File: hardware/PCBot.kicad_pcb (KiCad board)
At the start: 4 copper layers, 68 x 37 mm, 101 parts, among them J101 Conn_ST_STDC14, M101 Motor_DC_ALT, M102 Motor_DC_ALT, U101 STM32G431CBUx, U102 AMS1117-3.3, U103 LSM6DS3, U104 STSPIN250, U105 STSPIN250, U201 A7105, Y101 Crystal_GND24_DNP, Y201 Crystal_GND24_DNP

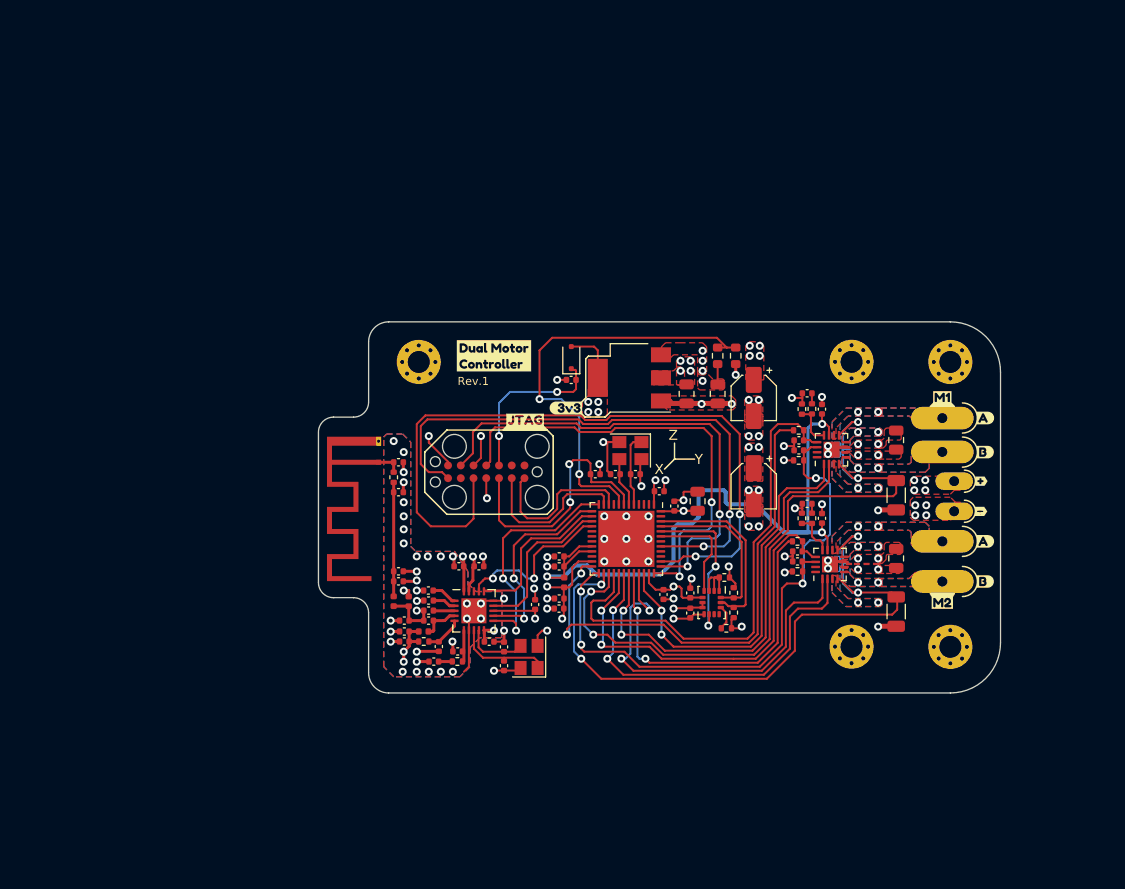
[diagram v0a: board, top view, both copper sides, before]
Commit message: initial commit 3
Signed-off-by: Connor Rigby <connorr@hey.com>
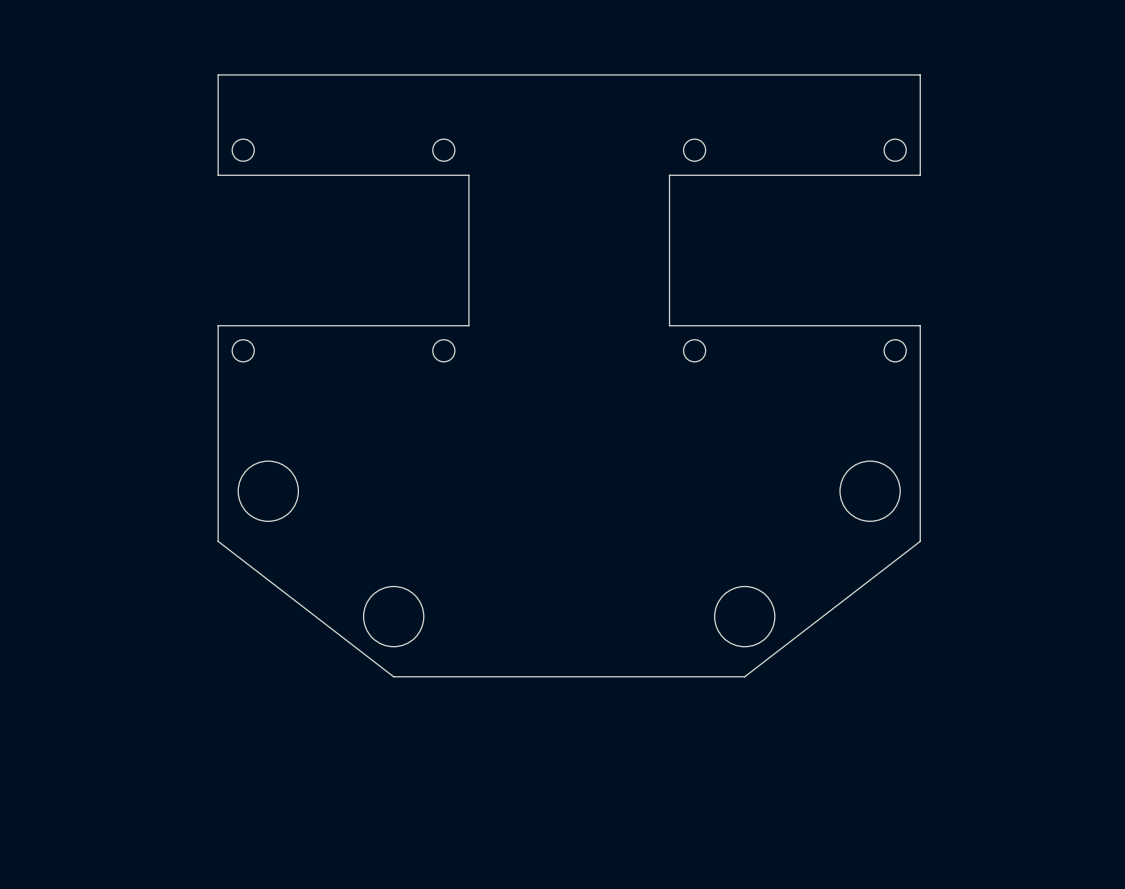
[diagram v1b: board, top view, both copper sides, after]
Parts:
- removed AE201: Antenna_Chip, RF_Antenna:Texas_SWRA117D_2.4GHz_Left
- removed BT101: Battery, LCSC_Connector:PAD_01x02
- removed C101, C102, C103, C109, C110, C114, C127, C128, C203, C206, C207, C208, C209, C211, C214, C215, C216, C217, C218, C219, C220: C_0402_DNP, Capacitor_SMD:C_0402_1005Metric
- removed C104, C111: C_0402_1nf_X7R, Capacitor_SMD:C_0402_1005Metric
- removed C105, C112: C_805_DNP, Capacitor_SMD:C_0805_2012Metric
- removed C106, C113: 22uf, Capacitor_SMD:CP_Elec_4x5.4
- removed C107: C_0805_1u_X7R, Capacitor_SMD:C_0805_2012Metric
- removed C108: C_0805_10u_X5R, Capacitor_SMD:C_0805_2012Metric
- removed C115, C116, C117, C118, C119, C122, C123, C124, C125, C126, C205: C_0402_100nf_X7R, Capacitor_SMD:C_0402_1005Metric
- removed C120: C_0805_4u7_X5R, Capacitor_SMD:C_0805_2012Metric
- removed C121: C_0402_1u_X5R, Capacitor_SMD:C_0402_1005Metric
- removed C201, C202, C204: C_0402_2u2_X5R, Capacitor_SMD:C_0402_1005Metric
- removed C210: C_0402_22p_C0G, Capacitor_SMD:C_0402_1005Metric
- removed C212: C_0402_100p_C0G, Capacitor_SMD:C_0402_1005Metric
- removed C213: C_0402_10n_C0G, Capacitor_SMD:C_0402_1005Metric
- removed D101: 30v 230mv@100ma 1A, Diode_SMD:D_SOD-323F
- removed FB101: FerriteBead_Small, Inductor_SMD:L_0402_1005Metric
- removed J101: Conn_ST_STDC14, LCSC_Connector:TC2070-IDC-FP
- removed L202, L203, L204: L_0402_DNP, Inductor_SMD:L_0402_1005Metric
- removed M101, M102: Motor_DC_ALT, LCSC_Connector:PAD_01x02
- removed R101, R102, R103, R106, R107, R110: 18k, Resistor_SMD:R_0402_1005Metric
- removed R104, R109, R113, R116: R_0402_1k, Resistor_SMD:R_0402_1005Metric
- removed R105, R108: R_1206_DNP, Resistor_SMD:R_1206_3216Metric
- removed R111, R112: R_0603_DNP, Resistor_SMD:R_0603_1608Metric
- removed R114, R115: R_0402_4k7, Resistor_SMD:R_0402_1005Metric
- removed R201, R203: DNP, Resistor_SMD:R_0402_1005Metric
- removed R202: 200, Resistor_SMD:R_0402_1005Metric
- removed REF** (x5): MountingHole_2.2mm_M2_Pad_Via, MountingHole:MountingHole_2.2mm_M2_Pad_Via
- removed U101: STM32G431CBUx, Package_DFN_QFN:QFN-48-1EP_7x7mm_P0.5mm_EP5.6x5.6mm
- removed U102: AMS1117-3.3, Package_TO_SOT_SMD:SOT-223-3_TabPin2
- removed U103: LSM6DS3, Package_LGA:LGA-14_3x2.5mm_P0.5mm_LayoutBorder3x4y
- removed U104, U105: STSPIN250, Package_DFN_QFN:TQFN-16-1EP_3x3mm_P0.5mm_EP1.6x1.6mm
- removed U201: A7105, Package_DFN_QFN:QFN-20-1EP_4x4mm_P0.5mm_EP2.5x2.5mm
- removed Y101, Y201: Crystal_GND24_DNP, Crystal:Crystal_SMD_3225-4Pin_3.2x2.5mm
- removed kibuzzard-646A62D2: G***, kibuzzard-646A62D2
- removed kibuzzard-646A6321: G***, kibuzzard-646A6321
- removed kibuzzard-646A63AE (x2): G***, kibuzzard-646A63AE
- removed kibuzzard-646A6533 (x2): G***, kibuzzard-646A6533
- removed kibuzzard-646A657B (x2): G***, kibuzzard-646A657B
- removed kibuzzard-646A6855: G***, kibuzzard-646A6855
- removed kibuzzard-646A6AA4: G***, kibuzzard-646A6AA4
- removed kibuzzard-646A6DD1: G***, kibuzzard-646A6DD1
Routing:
- net GND: track 90.8 -> 0.00 mm, vias 95 -> 0
- net /SYS_JTDI: track 72.9 -> 0.00 mm, vias 2 -> 0
- net /M2_SENSE: track 70.6 -> 0.00 mm, vias 4 -> 0
- net VDDA: track 67.8 -> 0.00 mm, vias 3 -> 0
- net /M1_SENSE: track 66.1 -> 0.00 mm, vias 4 -> 0
- net /MC_STBY_RESET: track 60.4 -> 0.00 mm, vias 4 -> 0
- net /SYS_JTDO: track 56.8 -> 0.00 mm, vias 2 -> 0
- net /M2_EN: track 51.9 -> 0.00 mm, vias 2 -> 0
- net /M2_EN_FAULT: track 50.7 -> 0.00 mm
- net VDD: track 48.6 -> 0.00 mm, vias 20 -> 0
- net /SYS_JTCK: track 48.2 -> 0.00 mm, vias 2 -> 0
- net /SYS_JTMS: track 45.8 -> 0.00 mm, vias 2 -> 0
- net /M2_PWM: track 43.6 -> 0.00 mm, vias 2 -> 0
- net /VBATT_SENSE: track 42.9 -> 0.00 mm, vias 2 -> 0
- net /M1_EN_FAULT: track 41.8 -> 0.00 mm, vias 2 -> 0
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- removed copper zone on F.Cu, net +BATT
- removed copper zone on B.Cu, net /M1_OUTA1
- removed copper zone on F.Cu, net /M1_OUTA1
- removed copper zone on B.Cu, net /M1_OUTA2
- removed copper zone on F.Cu, net /M1_OUTA2
- removed copper zone on B.Cu, net /M2_OUTA1
- removed copper zone on F.Cu, net /M2_OUTA1
- removed copper zone on B.Cu, net /M2_OUTA2
- removed copper zone on F.Cu, net /M2_OUTA2
- removed copper zone on B.Cu, net GND
- removed copper zone on F.Cu, net GND
- removed copper zone on F.Cu, net VDD
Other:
- board size 68 x 37 mm -> 70 x 60 mm
- board text removed: "Rev.1"
- board text removed: "X"
- board text removed: "Y"
- board text removed: "Z"

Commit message: uhhhhhhhhhhhhhhhhhhhhhhhh
Signed-off-by: Connor Rigby <connorr@hey.com>
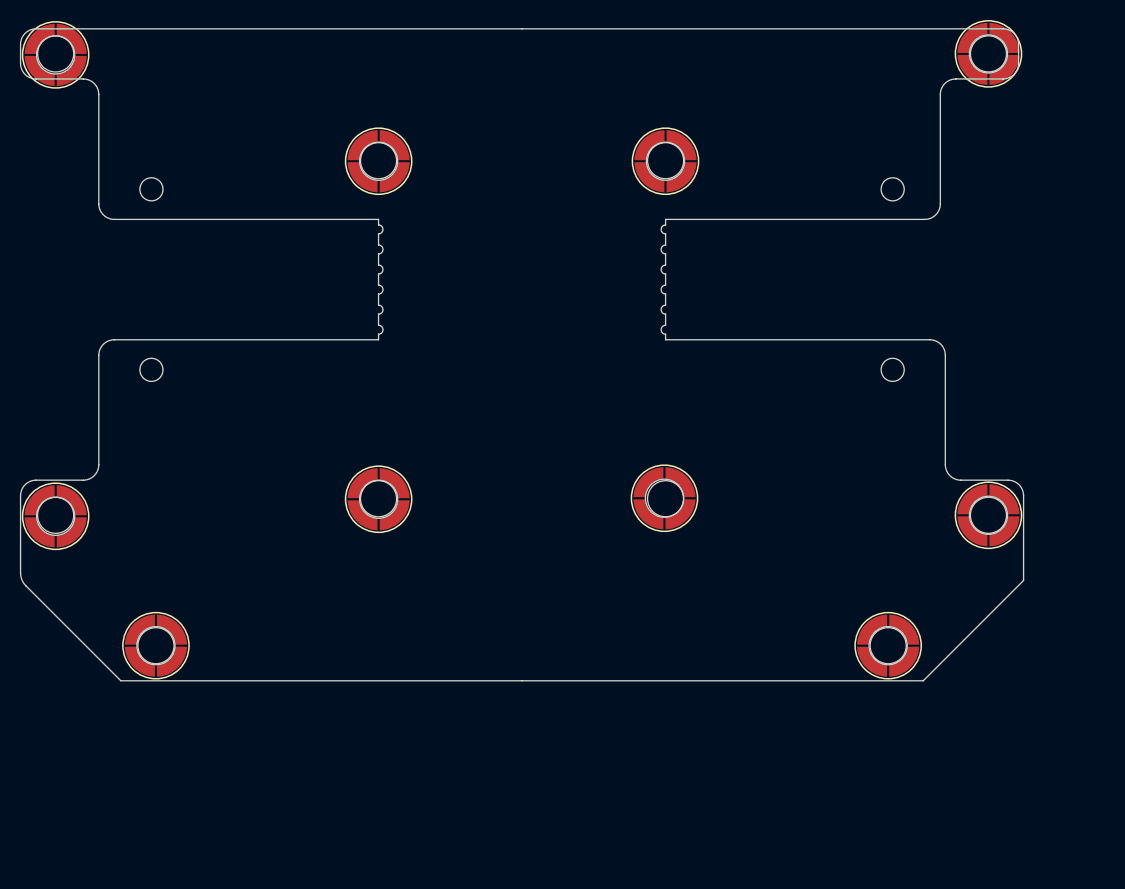
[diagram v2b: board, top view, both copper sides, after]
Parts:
- added REF**: SMD_BD5.6-L5.6-W5.6-D3.6, LCSC_Connector:SMD_BD5.6-L5.6-W5.6-D3.6, F.Cu at (116.8, 22.9)
- added REF**: SMD_BD5.6-L5.6-W5.6-D3.6, LCSC_Connector:SMD_BD5.6-L5.6-W5.6-D3.6, F.Cu at (84.5, 67.2)
- added REF**: SMD_BD5.6-L5.6-W5.6-D3.6, LCSC_Connector:SMD_BD5.6-L5.6-W5.6-D3.6, F.Cu at (23.8, 69.0)
- added REF**: SMD_BD5.6-L5.6-W5.6-D3.6, LCSC_Connector:SMD_BD5.6-L5.6-W5.6-D3.6, F.Cu at (56.0, 33.6)
- added REF**: SMD_BD5.6-L5.6-W5.6-D3.6, LCSC_Connector:SMD_BD5.6-L5.6-W5.6-D3.6, F.Cu at (56.0, 67.3)
- added REF**: SMD_BD5.6-L5.6-W5.6-D3.6, LCSC_Connector:SMD_BD5.6-L5.6-W5.6-D3.6, F.Cu at (33.8, 81.9)
- added REF**: SMD_BD5.6-L5.6-W5.6-D3.6, LCSC_Connector:SMD_BD5.6-L5.6-W5.6-D3.6, F.Cu at (84.6, 33.6)
- added REF**: SMD_BD5.6-L5.6-W5.6-D3.6, LCSC_Connector:SMD_BD5.6-L5.6-W5.6-D3.6, F.Cu at (116.8, 68.9)
- added REF**: SMD_BD5.6-L5.6-W5.6-D3.6, LCSC_Connector:SMD_BD5.6-L5.6-W5.6-D3.6, F.Cu at (23.8, 23.0)
- added REF**: SMD_BD5.6-L5.6-W5.6-D3.6, LCSC_Connector:SMD_BD5.6-L5.6-W5.6-D3.6, F.Cu at (106.8, 81.9)
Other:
- board size 70 x 60 mm -> 100 x 65 mm

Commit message: initial commit 69
Signed-off-by: Connor Rigby <connorr@hey.com>
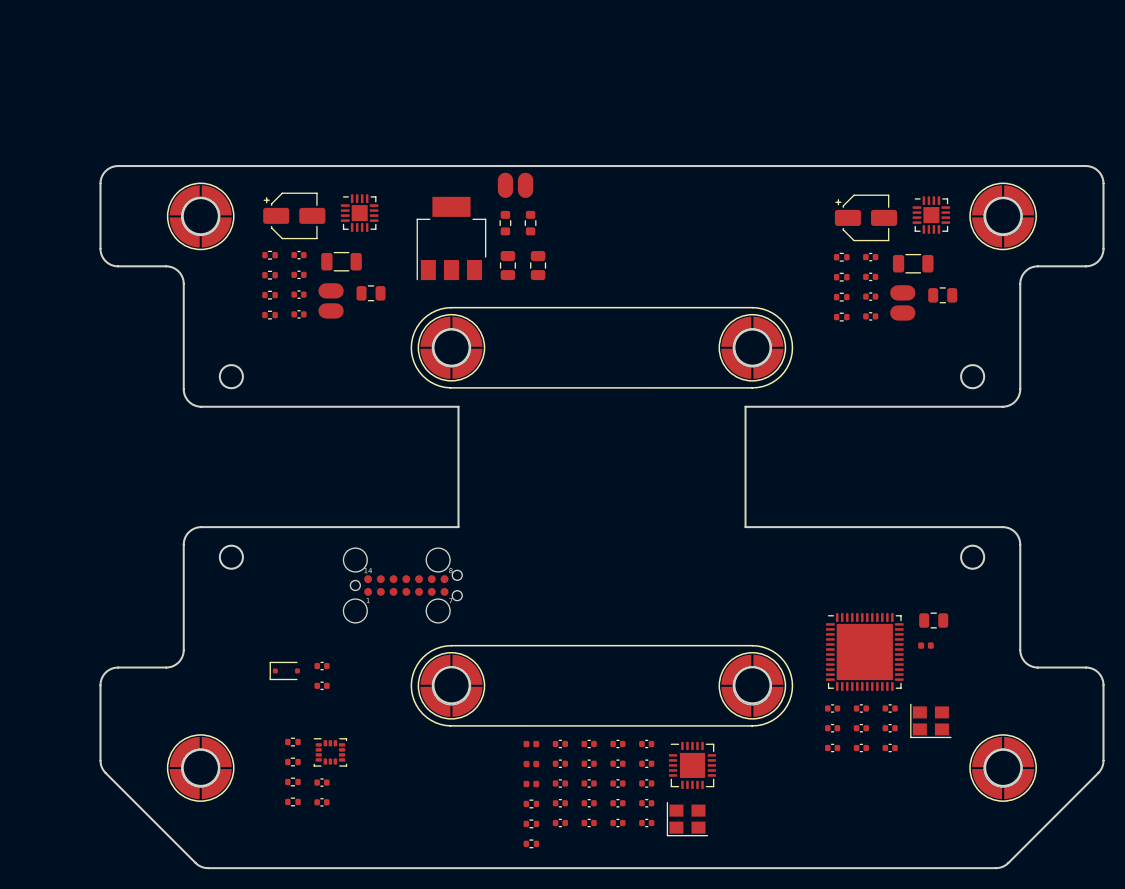
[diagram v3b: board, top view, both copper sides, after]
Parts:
- removed the REF** at (116.8, 22.9)
- removed the REF** at (84.5, 67.2)
- removed the REF** at (23.8, 69.0)
- removed the REF** at (56.0, 33.6)
- removed the REF** at (56.0, 67.3)
- removed the REF** at (33.8, 81.9)
- removed the REF** at (84.6, 33.6)
- removed the REF** at (116.8, 68.9)
- removed the REF** at (23.8, 23.0)
- removed the REF** at (106.8, 81.9)
- added BT101: Battery, LCSC_Connector:PAD_01x02, F.Cu at (68.6, 36.0)
- added C101: C_0402_DNP, Capacitor_SMD:C_0402_1005Metric, F.Cu at (105.1, 43.2)
- added C102: C_0402_DNP, Capacitor_SMD:C_0402_1005Metric, F.Cu at (105.1, 45.1)
- added C103: C_0402_DNP, Capacitor_SMD:C_0402_1005Metric, F.Cu at (105.1, 47.1)
- added C104: C_0402_1nf_X7R, Capacitor_SMD:C_0402_1005Metric, F.Cu at (105.1, 49.1)
- added C105: C_805_DNP, Capacitor_SMD:C_0805_2012Metric, F.Cu at (112.2, 47.0)
- added C106: 22uf, Capacitor_SMD:CP_Elec_4x5.4, F.Cu at (104.6, 39.2)
- added C107: C_0805_1u_X7R, Capacitor_SMD:C_0805_2012Metric, F.Cu at (68.9, 44.0)
- added C108: C_0805_10u_X5R, Capacitor_SMD:C_0805_2012Metric, F.Cu at (71.9, 44.0)
- added C109: C_0402_DNP, Capacitor_SMD:C_0402_1005Metric, F.Cu at (48.1, 43.0)
- added C110: C_0402_DNP, Capacitor_SMD:C_0402_1005Metric, F.Cu at (48.1, 44.9)
- added C111: C_0402_1nf_X7R, Capacitor_SMD:C_0402_1005Metric, F.Cu at (48.1, 46.9)
- added C112: C_805_DNP, Capacitor_SMD:C_0805_2012Metric, F.Cu at (55.2, 46.8)
- added C113: 22uf, Capacitor_SMD:CP_Elec_4x5.4, F.Cu at (47.6, 39.0)
- added C114: C_0402_DNP, Capacitor_SMD:C_0402_1005Metric, F.Cu at (48.1, 48.9)
- added C115: C_0402_100nf_X7R, Capacitor_SMD:C_0402_1005Metric, F.Cu at (101.3, 88.2)
- added C116: C_0402_100nf_X7R, Capacitor_SMD:C_0402_1005Metric, F.Cu at (101.3, 90.1)
- added C117: C_0402_100nf_X7R, Capacitor_SMD:C_0402_1005Metric, F.Cu at (101.3, 92.1)
- added C118: C_0402_100nf_X7R, Capacitor_SMD:C_0402_1005Metric, F.Cu at (104.1, 88.2)
- added C119: C_0402_100nf_X7R, Capacitor_SMD:C_0402_1005Metric, F.Cu at (104.1, 90.1)
- added C120: C_0805_4u7_X5R, Capacitor_SMD:C_0805_2012Metric, F.Cu at (111.3, 79.4)
- added C121: C_0402_1u_X5R, Capacitor_SMD:C_0402_1005Metric, F.Cu at (104.1, 92.1)
- added C122: C_0402_100nf_X7R, Capacitor_SMD:C_0402_1005Metric, F.Cu at (107.0, 88.2)
- added C123: C_0402_100nf_X7R, Capacitor_SMD:C_0402_1005Metric, F.Cu at (50.4, 83.9)
- added C124: C_0402_100nf_X7R, Capacitor_SMD:C_0402_1005Metric, F.Cu at (50.4, 85.9)
- added C125: C_0402_100nf_X7R, Capacitor_SMD:C_0402_1005Metric, F.Cu at (50.4, 95.5)
- added C126: C_0402_100nf_X7R, Capacitor_SMD:C_0402_1005Metric, F.Cu at (50.4, 97.5)
- added C127: C_0402_DNP, Capacitor_SMD:C_0402_1005Metric, F.Cu at (107.0, 90.1)
- added C128: C_0402_DNP, Capacitor_SMD:C_0402_1005Metric, F.Cu at (107.0, 92.1)
- added C201: C_0402_2u2_X5R, Capacitor_SMD:C_0402_1005Metric, F.Cu at (74.1, 91.7)
- added C202: C_0402_2u2_X5R, Capacitor_SMD:C_0402_1005Metric, F.Cu at (74.1, 93.7)
- added C203: C_0402_DNP, Capacitor_SMD:C_0402_1005Metric, F.Cu at (74.1, 95.6)
- added C204: C_0402_2u2_X5R, Capacitor_SMD:C_0402_1005Metric, F.Cu at (74.1, 97.6)
- added C205: C_0402_100nf_X7R, Capacitor_SMD:C_0402_1005Metric, F.Cu at (74.1, 99.6)
- added C206: C_0402_DNP, Capacitor_SMD:C_0402_1005Metric, F.Cu at (77.0, 91.7)
- added C207: C_0402_DNP, Capacitor_SMD:C_0402_1005Metric, F.Cu at (77.0, 93.7)
- added C208: C_0402_DNP, Capacitor_SMD:C_0402_1005Metric, F.Cu at (77.0, 95.6)
- added C209: C_0402_DNP, Capacitor_SMD:C_0402_1005Metric, F.Cu at (77.0, 97.6)
- added C210: C_0402_22p_C0G, Capacitor_SMD:C_0402_1005Metric, F.Cu at (77.0, 99.6)
- added C211: C_0402_DNP, Capacitor_SMD:C_0402_1005Metric, F.Cu at (79.9, 91.7)
- added C212: C_0402_100p_C0G, Capacitor_SMD:C_0402_1005Metric, F.Cu at (79.9, 93.7)
- added C213: C_0402_10n_C0G, Capacitor_SMD:C_0402_1005Metric, F.Cu at (79.9, 95.6)
- added C214: C_0402_DNP, Capacitor_SMD:C_0402_1005Metric, F.Cu at (79.9, 97.6)
- added C215: C_0402_DNP, Capacitor_SMD:C_0402_1005Metric, F.Cu at (79.9, 99.6)
- added C216: C_0402_DNP, Capacitor_SMD:C_0402_1005Metric, F.Cu at (82.7, 91.7)
- added C217: C_0402_DNP, Capacitor_SMD:C_0402_1005Metric, F.Cu at (82.7, 93.7)
- added C218: C_0402_DNP, Capacitor_SMD:C_0402_1005Metric, F.Cu at (82.7, 95.6)
- added C219: C_0402_DNP, Capacitor_SMD:C_0402_1005Metric, F.Cu at (82.7, 97.6)
- added C220: C_0402_DNP, Capacitor_SMD:C_0402_1005Metric, F.Cu at (82.7, 99.6)
- added D101: 30v 230mv@100ma 1A, Diode_SMD:D_SOD-323F, F.Cu at (46.8, 84.4)
- added FB101: FerriteBead_Small, Inductor_SMD:L_0402_1005Metric, F.Cu at (110.6, 81.9)
- added J101: Conn_ST_STDC14, LCSC_Connector:TC2070-IDC-FP, F.Cu at (58.8, 75.9)
- added L202: L_0402_DNP, Inductor_SMD:L_0402_1005Metric, F.Cu at (71.2, 91.7)
- added L203: L_0402_DNP, Inductor_SMD:L_0402_1005Metric, F.Cu at (71.2, 93.7)
- added L204: L_0402_DNP, Inductor_SMD:L_0402_1005Metric, F.Cu at (71.2, 95.7)
- added M101: Motor_DC_ALT, LCSC_Connector:PAD_01x02, F.Cu at (108.3, 46.7)
- added M102: Motor_DC_ALT, LCSC_Connector:PAD_01x02, F.Cu at (51.3, 46.5)
- added R101: 18k, Resistor_SMD:R_0402_1005Metric, F.Cu at (102.2, 43.2)
- added R102: 18k, Resistor_SMD:R_0402_1005Metric, F.Cu at (102.2, 45.2)
- added R103: 18k, Resistor_SMD:R_0402_1005Metric, F.Cu at (102.2, 47.1)
- added R104: R_0402_1k, Resistor_SMD:R_0402_1005Metric, F.Cu at (102.2, 49.1)
- added R105: R_1206_DNP, Resistor_SMD:R_1206_3216Metric, F.Cu at (109.3, 43.8)
- added R106: 18k, Resistor_SMD:R_0402_1005Metric, F.Cu at (45.2, 43.0)
- added R107: 18k, Resistor_SMD:R_0402_1005Metric, F.Cu at (45.2, 45.0)
- added R108: R_1206_DNP, Resistor_SMD:R_1206_3216Metric, F.Cu at (52.3, 43.6)
- added R109: R_0402_1k, Resistor_SMD:R_0402_1005Metric, F.Cu at (45.2, 47.0)
- added R110: 18k, Resistor_SMD:R_0402_1005Metric, F.Cu at (45.2, 48.9)
- added R111: R_0603_DNP, Resistor_SMD:R_0603_1608Metric, F.Cu at (68.6, 39.8)
- added R112: R_0603_DNP, Resistor_SMD:R_0603_1608Metric, F.Cu at (71.2, 39.8)
- added R113: R_0402_1k, Resistor_SMD:R_0402_1005Metric, F.Cu at (47.5, 91.5)
- added R114: R_0402_4k7, Resistor_SMD:R_0402_1005Metric, F.Cu at (47.5, 93.5)
- added R115: R_0402_4k7, Resistor_SMD:R_0402_1005Metric, F.Cu at (47.5, 95.5)
- added R116: R_0402_1k, Resistor_SMD:R_0402_1005Metric, F.Cu at (47.5, 97.5)
- added R201: DNP, Resistor_SMD:R_0402_1005Metric, F.Cu at (71.2, 97.7)
- added R202: 200, Resistor_SMD:R_0402_1005Metric, F.Cu at (71.2, 99.7)
- added R203: DNP, Resistor_SMD:R_0402_1005Metric, F.Cu at (71.2, 101.7)
- added REF**: SMD_BD5.6-L5.6-W5.6-D3.6, LCSC_Connector:SMD_BD5.6-L5.6-W5.6-D3.6, F.Cu at (93.3, 85.9)
- added REF**: SMD_BD5.6-L5.6-W5.6-D3.6, LCSC_Connector:SMD_BD5.6-L5.6-W5.6-D3.6, F.Cu at (63.3, 52.2)
- added REF**: SMD_BD5.6-L5.6-W5.6-D3.6, LCSC_Connector:SMD_BD5.6-L5.6-W5.6-D3.6, F.Cu at (118.3, 39.1)
- added REF**: SMD_BD5.6-L5.6-W5.6-D3.6, LCSC_Connector:SMD_BD5.6-L5.6-W5.6-D3.6, F.Cu at (63.3, 85.9)
- added REF**: SMD_BD5.6-L5.6-W5.6-D3.6, LCSC_Connector:SMD_BD5.6-L5.6-W5.6-D3.6, F.Cu at (38.3, 39.1)
- added REF**: SMD_BD5.6-L5.6-W5.6-D3.6, LCSC_Connector:SMD_BD5.6-L5.6-W5.6-D3.6, F.Cu at (93.3, 52.2)
- added REF**: SMD_BD5.6-L5.6-W5.6-D3.6, LCSC_Connector:SMD_BD5.6-L5.6-W5.6-D3.6, F.Cu at (38.3, 94.1)
- added REF**: SMD_BD5.6-L5.6-W5.6-D3.6, LCSC_Connector:SMD_BD5.6-L5.6-W5.6-D3.6, F.Cu at (118.3, 94.1)
- added U101: STM32G431CBUx, Package_DFN_QFN:QFN-48-1EP_7x7mm_P0.5mm_EP5.6x5.6mm, F.Cu at (104.5, 82.5)
- added U102: AMS1117-3.3, Package_TO_SOT_SMD:SOT-223-3_TabPin2, F.Cu at (63.3, 41.3)
- added U103: LSM6DS3, Package_LGA:LGA-14_3x2.5mm_P0.5mm_LayoutBorder3x4y, F.Cu at (51.2, 92.5)
- added U104: STSPIN250, Package_DFN_QFN:TQFN-16-1EP_3x3mm_P0.5mm_EP1.6x1.6mm, F.Cu at (111.1, 39.0)
- added U105: STSPIN250, Package_DFN_QFN:TQFN-16-1EP_3x3mm_P0.5mm_EP1.6x1.6mm, F.Cu at (54.1, 38.8)
- added U201: A7105, Package_DFN_QFN:QFN-20-1EP_4x4mm_P0.5mm_EP2.5x2.5mm, F.Cu at (87.3, 93.8)
- added Y101: Crystal_GND24_DNP, Crystal:Crystal_SMD_3225-4Pin_3.2x2.5mm, F.Cu at (111.1, 89.4)
- added Y201: Crystal_GND24_DNP, Crystal:Crystal_SMD_3225-4Pin_3.2x2.5mm, F.Cu at (86.8, 99.2)
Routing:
- removed copper zone on In2.Cu, net +BATT
- removed copper zone on In2.Cu, net /RF_Transciever/REG0A
- removed copper zone on In1.Cu, net GND
- removed copper zone on In2.Cu, net VDD
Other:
- board size 100 x 65 mm -> 100 x 70 mm
- copper layers 4 -> 2
